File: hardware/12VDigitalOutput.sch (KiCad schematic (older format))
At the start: 6 parts, among them Q2701 ZXTN25050DFHTA, Q2702 ZXTN25050DFHTA

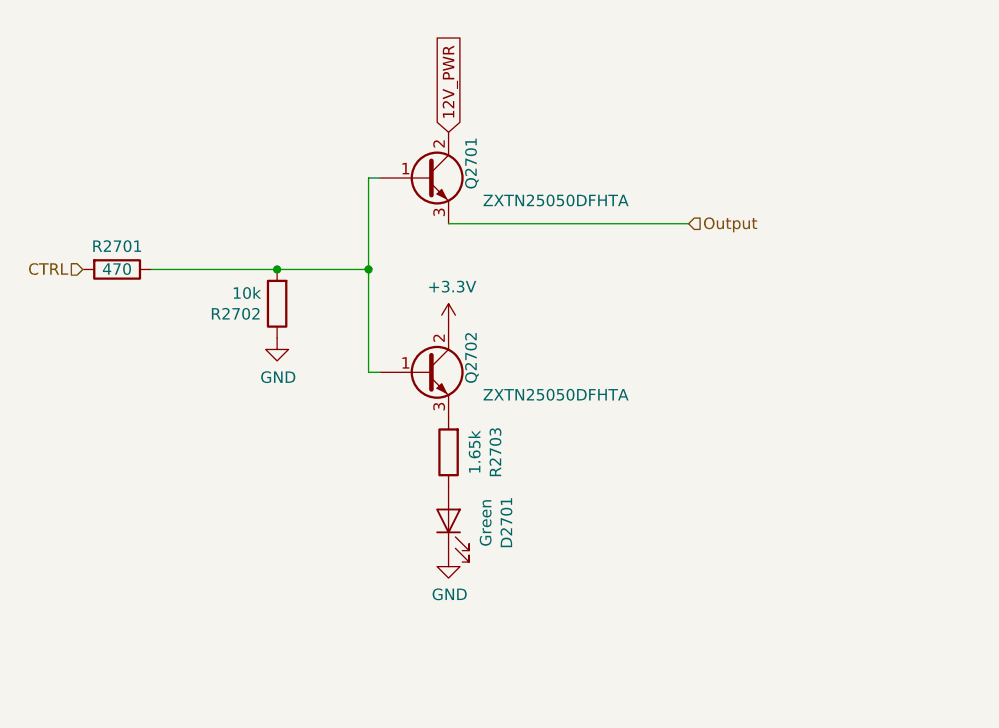
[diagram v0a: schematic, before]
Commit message: Outputs now uses MOSFETs
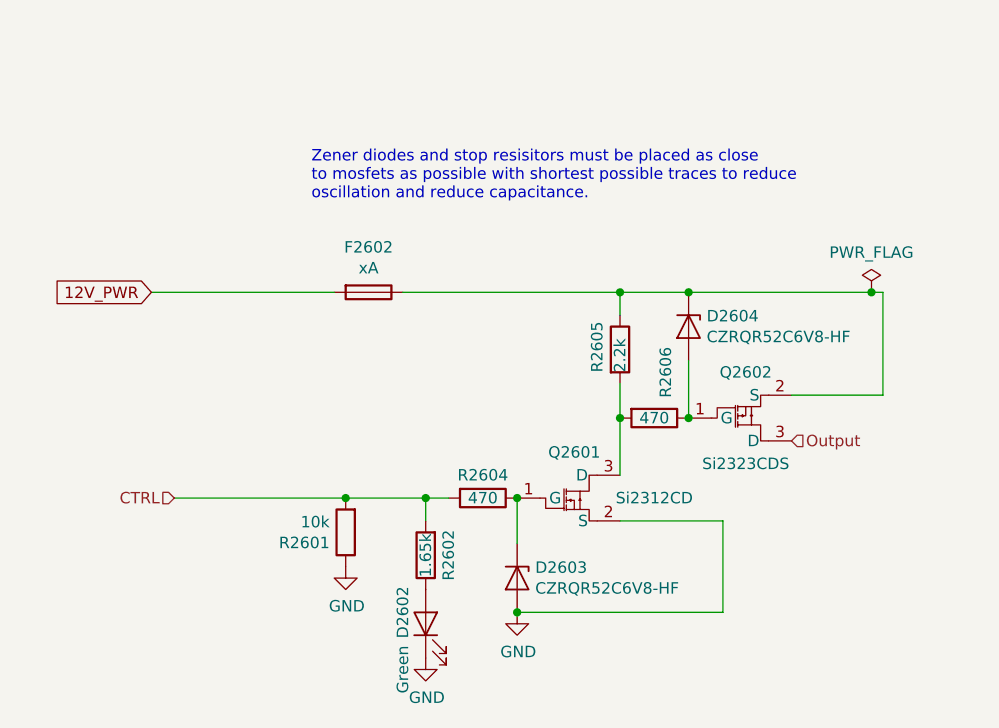
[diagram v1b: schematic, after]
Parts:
- removed D2701: Green, LED_THT:LED_D5.0mm, symbol Device:LED
- removed Q2701, Q2702: ZXTN25050DFHTA, Package_TO_SOT_SMD:SOT-23, symbol Device:Q_NPN_BCE
- removed R2701: 470, Resistor_SMD:R_0805_2012Metric, symbol Device:R
- removed R2702: 10k, Resistor_SMD:R_0805_2012Metric, symbol Device:R
- removed R2703: 1.65k, Resistor_SMD:R_0805_2012Metric, symbol Device:R
- added D2602: Green, LED_THT:LED_D5.0mm, symbol Device:LED
- added D2603, D2604: CZRQR52C6V8-HF, Diode_SMD:D_0402_1005Metric, symbol Device:D_Zener
- added F2602: xA, Fuse:Fuseholder_TR5_Littlefuse_No560_No460, symbol Device:Fuse
- added Q2601: Si2312CD, Package_TO_SOT_SMD:SOT-23, symbol PerMalmberg:Si2312CD
- added Q2602: Si2323CDS, Package_TO_SOT_SMD:SOT-23, symbol PerMalmberg:Si2323CDS
- added R2601: 10k, Resistor_SMD:R_0805_2012Metric, symbol Device:R
- added R2602: 1.65k, Resistor_SMD:R_0805_2012Metric, symbol Device:R
- added R2604, R2606: 470, Resistor_SMD:R_0805_2012Metric, symbol Device:R
- added R2605: 2.2k, symbol Device:R
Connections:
- net 12V_PWR: now also F2602.2
- net CTRL: now also R2601.2, R2602.2, R2604.2
- net GND: now also D2602.1 (K), D2603.2 (A), Q2601.2 (S), R2601.1
- net Output: now also Q2602.3 (D)
- new net: D2604.1 (K), F2602.1, Q2602.2 (S), R2605.1
- new net: D2602.2 (A), R2602.1
- new net: D2603.1 (K), Q2601.1 (G), R2604.1
- new net: Q2601.3 (D), R2605.2, R2606.2
- new net: D2604.2 (A), Q2602.1 (G), R2606.1
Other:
- note added: "Zener diodes and stop resisitors must be placed as close\nto mosfets as possible with shortest possible traces to reduce\noscillation and reduce capacitance."

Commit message: Preparing to replicate layout for outputs.
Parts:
- F2602: footprint Fuse:Fuseholder_TR5_Littlefuse_No560_No460 -> Fuse:Fuseholder_TR5_Littelfuse_No560_No460
- R2605: footprint (none) -> Resistor_SMD:R_0805_2012Metric
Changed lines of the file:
@@
 F 0 "F2602" V 3103 2350 50  0000 C CNN
 F 1 "xA" V 3194 2350 50  0000 C CNN
-F 2 "Fuse:Fuseholder_TR5_Littlefuse_No560_No460" V 3230 2350 50  0001 C CNN
+F 2 "Fuse:Fuseholder_TR5_Littelfuse_No560_No460" V 3230 2350 50  0001 C CNN
 F 3 "https://www.mouser.se/ProductDetail/Littelfuse/56000001019?qs=sGAEpiMZZMtRmoYvq3OwzKEcK5xXAR8uiSqvDZfRA1w%3d" H 3300 2350 50  0001 C CNN
 	1    3300 2350
@@
 F 1 "470" V 4550 2900 50  0000 C CNN
 F 2 "Resistor_SMD:R_0805_2012Metric" V 4480 2900 50  0001 C CNN
-F 3 "~" H 4550 2900 50  0001 C CNN
+F 3 "https://www.mouser.se/ProductDetail/Yageo/RT0805FRE07470RL?qs=sGAEpiMZZMu61qfTUdNhG7XKrGAE6fxHsvRUjrIFZAo%3d" H 4550 2900 50  0001 C CNN
 	1    4550 2900
 	0    1    1    0
@@
 F 0 "R2605" V 4300 2500 50  0000 L CNN
 F 1 "2.2k" V 4400 2500 50  0000 L CNN
-F 2 "" V 4330 2600 50  0001 C CNN
-F 3 "~" H 4400 2600 50  0001 C CNN
+F 2 "Resistor_SMD:R_0805_2012Metric" V 4330 2600 50  0001 C CNN
+F 3 "https://www.mouser.se/ProductDetail/Panasonic/ERA-6AED222V?qs=sGAEpiMZZMu61qfTUdNhGxFN6bFILsDSLGMUiuxodHY%3d" H 4400 2600 50  0001 C CNN
 	1    4400 2600
 	1    0    0    -1
